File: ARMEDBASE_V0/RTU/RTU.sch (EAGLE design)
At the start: 27 parts, among them IC1 REG1117, IC2 MEGA8-P, Q1 20Mhz, Q2 2N3904

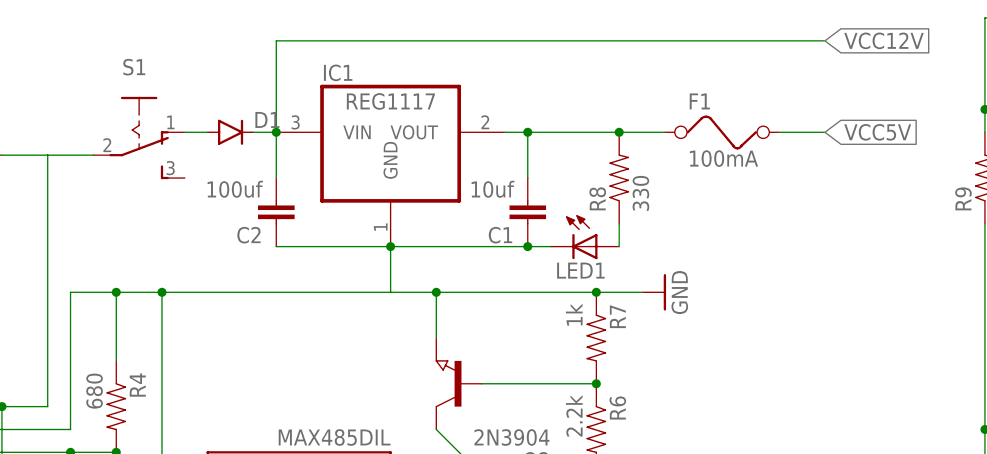
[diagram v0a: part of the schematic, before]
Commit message: rtu fuse
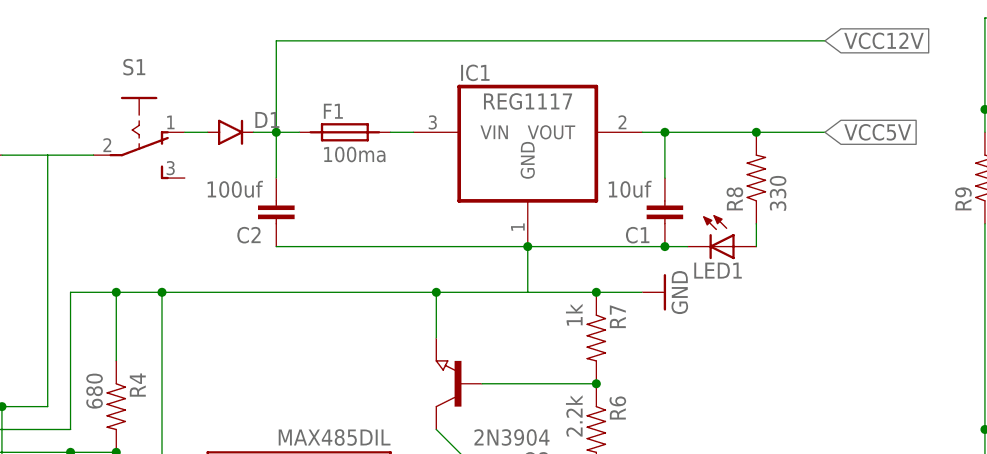
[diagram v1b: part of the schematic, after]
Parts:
- F1: value 100mA -> 100ma; device special:FUSE -> _hhn_PtcFuses_Siba_r500_Ozan:SIBA194600
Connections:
- net N$9: now also F1.2, IC1.VIN; no longer C1.2, F1.1, IC1.VOUT, R8.2
- net VCC12V: now also F1.1; no longer IC1.VIN
- net VCC5V: now also C1.2, IC1.VOUT, R8.2; no longer F1.2
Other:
- moved on the sheet: C1, IC1, LED1, R8
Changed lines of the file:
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@@
 </variantdefs>
 <classes>
-<class number="0" name="default" width="0" drill="0">
+<class number="0" name="default" width="0.3" drill="0.5">
+<clearance class="0" value="0.25"/>
 </class>
 </classes>
@@
 <part name="R8" library="SparkFun-Passives" deviceset="RESISTOR" device="0805-RES" value="330"/>
 <part name="P&amp;C1" library="con-4ucon" deviceset="14867" device=""/>
-<part name="F1" library="special" deviceset="FUSE" device="" value="100mA"/>
+<part name="F1" library="_hhn_PtcFuses_Siba_r500_Ozan" deviceset="SIBA194600*" device="" value="100ma"/>
 </parts>
 <sheets>
@@
 <instance part="LOGO1" gate="G$1" x="134.62" y="22.86"/>
 <instance part="S2" gate="G$1" x="137.16" y="76.2"/>
-<instance part="IC1" gate="G$1" x="60.96" y="73.66"/>
-<instance part="C1" gate="G$1" x="76.2" y="66.04" rot="R180"/>
-<instance part="LED1" gate="G$1" x="83.82" y="60.96" rot="R270"/>
+<instance part="IC1" gate="G$1" x="76.2" y="73.66"/>
+<instance part="C1" gate="G$1" x="91.44" y="66.04" rot="R180"/>
+<instance part="LED1" gate="G$1" x="99.06" y="60.96" rot="R270"/>
 <instance part="D1" gate="G$1" x="43.18" y="73.66"/>
 <instance part="SUPPLY1" gate="G$1" x="17.78" y="71.12" rot="R90"/>
 <instance part="S1" gate="1" x="33.02" y="73.66" rot="R270"/>
 <instance part="C2" gate="G$1" x="48.26" y="66.04" rot="R180"/>
-<instance part="R8" gate="G$1" x="86.36" y="68.58" rot="R90"/>
+<instance part="R8" gate="G$1" x="101.6" y="68.58" rot="R90"/>
 <instance part="P&amp;C1" gate="G$1" x="2.54" y="22.86" rot="R180"/>
-<instance part="F1" gate="G$1" x="99.06" y="73.66"/>
+<instance part="F1" gate="G$1" x="55.88" y="73.66"/>
 </instances>
 <busses>
@@
 </segment>
 <segment>
-<pinref part="F1" gate="G$1" pin="2"/>
-<wire x1="104.14" y1="73.66" x2="109.22" y2="73.66" width="0.1524" layer="91"/>
 <label x="109.22" y="73.66" size="1.778" layer="95" xref="yes"/>
+<pinref part="IC1" gate="G$1" pin="VOUT"/>
+<wire x1="88.9" y1="73.66" x2="91.44" y2="73.66" width="0.1524" layer="91"/>
+<pinref part="C1" gate="G$1" pin="2"/>
+<wire x1="91.44" y1="73.66" x2="91.44" y2="68.58" width="0.1524" layer="91"/>
+<wire x1="91.44" y1="73.66" x2="101.6" y2="73.66" width="0.1524" layer="91"/>
+<pinref part="R8" gate="G$1" pin="2"/>
+<junction x="101.6" y="73.66"/>
+<junction x="91.44" y="73.66"/>
+<wire x1="109.22" y1="73.66" x2="101.6" y2="73.66" width="0.1524" layer="91"/>
 </segment>
 </net>
 <net name="GND" class="0">
 <segment>
-<pinref part="Q2" gate="G$1" pin="E"/>
-<wire x1="66.04" y1="50.8" x2="66.04" y2="55.88" width="0.1524" layer="91"/>
 <pinref part="R7" gate="G$1" pin="1"/>
-<wire x1="66.04" y1="55.88" x2="83.82" y2="55.88" width="0.1524" layer="91"/>
+<wire x1="76.2" y1="55.88" x2="83.82" y2="55.88" width="0.1524" layer="91"/>
 <wire x1="83.82" y1="55.88" x2="88.9" y2="55.88" width="0.1524" layer="91"/>
 <junction x="83.82" y="55.88"/>
-<junction x="66.04" y="55.88"/>
-<wire x1="66.04" y1="55.88" x2="60.96" y2="55.88" width="0.1524" layer="91"/>
 <pinref part="U$1" gate="G$1" pin="GND"/>
-<wire x1="60.96" y1="55.88" x2="35.56" y2="55.88" width="0.1524" layer="91"/>
+<wire x1="76.2" y1="55.88" x2="66.04" y2="55.88" width="0.1524" layer="91"/>
+<wire x1="66.04" y1="55.88" x2="35.56" y2="55.88" width="0.1524" layer="91"/>
 <wire x1="35.56" y1="35.56" x2="35.56" y2="55.88" width="0.1524" layer="91"/>
 <junction x="35.56" y="55.88"/>
@@
 <pinref part="C2" gate="G$1" pin="1"/>
 <pinref part="IC1" gate="G$1" pin="GND"/>
-<wire x1="48.26" y1="60.96" x2="60.96" y2="60.96" width="0.1524" layer="91"/>
+<wire x1="48.26" y1="60.96" x2="76.2" y2="60.96" width="0.1524" layer="91"/>
 <pinref part="C1" gate="G$1" pin="1"/>
+<junction x="91.44" y="60.96"/>
+<wire x1="91.44" y1="60.96" x2="76.2" y2="60.96" width="0.1524" layer="91"/>
 <junction x="76.2" y="60.96"/>
-<wire x1="76.2" y1="60.96" x2="60.96" y2="60.96" width="0.1524" layer="91"/>
-<junction x="60.96" y="60.96"/>
 <pinref part="LED1" gate="G$1" pin="C"/>
-<wire x1="76.2" y1="60.96" x2="78.74" y2="60.96" width="0.1524" layer="91"/>
-<wire x1="60.96" y1="60.96" x2="60.96" y2="55.88" width="0.1524" layer="91"/>
+<wire x1="91.44" y1="60.96" x2="93.98" y2="60.96" width="0.1524" layer="91"/>
+<wire x1="76.2" y1="60.96" x2="76.2" y2="55.88" width="0.1524" layer="91"/>
 <wire x1="15.24" y1="40.64" x2="15.24" y2="22.86" width="0.1524" layer="91"/>
 <pinref part="P&amp;C1" gate="G$1" pin="3"/>
 <wire x1="15.24" y1="22.86" x2="5.08" y2="22.86" width="0.1524" layer="91"/>
 <junction x="15.24" y="40.64"/>
+<pinref part="Q2" gate="G$1" pin="E"/>
+<wire x1="66.04" y1="50.8" x2="66.04" y2="55.88" width="0.1524" layer="91"/>
+<junction x="66.04" y="55.88"/>
 </segment>
 <segment>
@@
 <segment>
 <pinref part="D1" gate="G$1" pin="C"/>
-<pinref part="IC1" gate="G$1" pin="VIN"/>
 <wire x1="45.72" y1="73.66" x2="48.26" y2="73.66" width="0.1524" layer="91"/>
 <pinref part="C2" gate="G$1" pin="2"/>
-<wire x1="48.26" y1="73.66" x2="48.26" y2="68.58" width="0.1524" layer="91"/>
-<junction x="48.26" y="73.66"/>
-<wire x1="48.26" y1="73.66" x2="48.26" y2="83.82" width="0.1524" layer="91"/>
+<wire x1="48.26" y1="73.66" x2="50.8" y2="73.66" width="0.1524" layer="91"/>
 <wire x1="48.26" y1="83.82" x2="109.22" y2="83.82" width="0.1524" layer="91"/>
 <label x="109.22" y="83.82" size="1.778" layer="95" xref="yes"/>
+<wire x1="48.26" y1="83.82" x2="48.26" y2="73.66" width="0.1524" layer="91"/>
+<wire x1="48.26" y1="68.58" x2="48.26" y2="73.66" width="0.1524" layer="91"/>
+<junction x="48.26" y="73.66"/>
+<pinref part="F1" gate="G$1" pin="1"/>
 </segment>
 </net>
@@
 <pinref part="R8" gate="G$1" pin="1"/>
 <pinref part="LED1" gate="G$1" pin="A"/>
-<wire x1="86.36" y1="60.96" x2="86.36" y2="63.5" width="0.1524" layer="91"/>
+<wire x1="101.6" y1="60.96" x2="101.6" y2="63.5" width="0.1524" layer="91"/>
 </segment>
 </net>
@@
 <net name="N$9" class="0">
 <segment>
-<pinref part="IC1" gate="G$1" pin="VOUT"/>
-<wire x1="73.66" y1="73.66" x2="76.2" y2="73.66" width="0.1524" layer="91"/>
-<pinref part="C1" gate="G$1" pin="2"/>
-<wire x1="76.2" y1="73.66" x2="76.2" y2="68.58" width="0.1524" layer="91"/>
-<wire x1="76.2" y1="73.66" x2="86.36" y2="73.66" width="0.1524" layer="91"/>
-<pinref part="R8" gate="G$1" pin="2"/>
-<wire x1="86.36" y1="73.66" x2="91.44" y2="73.66" width="0.1524" layer="91"/>
-<junction x="86.36" y="73.66"/>
-<junction x="76.2" y="73.66"/>
-<pinref part="F1" gate="G$1" pin="1"/>
-</segment>
-</net>
+<pinref part="IC1" gate="G$1" pin="VIN"/>
+<wire x1="60.96" y1="73.66" x2="63.5" y2="73.66" width="0.1524" layer="91"/>
+<pinref part="F1" gate="G$1" pin="2"/>
+</segment>
+</net>
